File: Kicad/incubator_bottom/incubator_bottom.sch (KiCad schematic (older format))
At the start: 42 parts, among them J1 Conn_01x02, J10 Conn_01x01, J11 Conn_01x01, J12 Conn_01x01, J2 Conn_02x03_Odd_Even, J3 RJ12, J4 Conn_01x01, J5 AudioJack3_SwitchTR, J6 AudioJack3_SwitchTR, J7 Conn_01x01, J8 Conn_01x06, J9 Conn_01x01, Q1 ZXMS6004, Q2 IPB80N03S4L-03, U1 DS18B20Z, U2 DS18B20

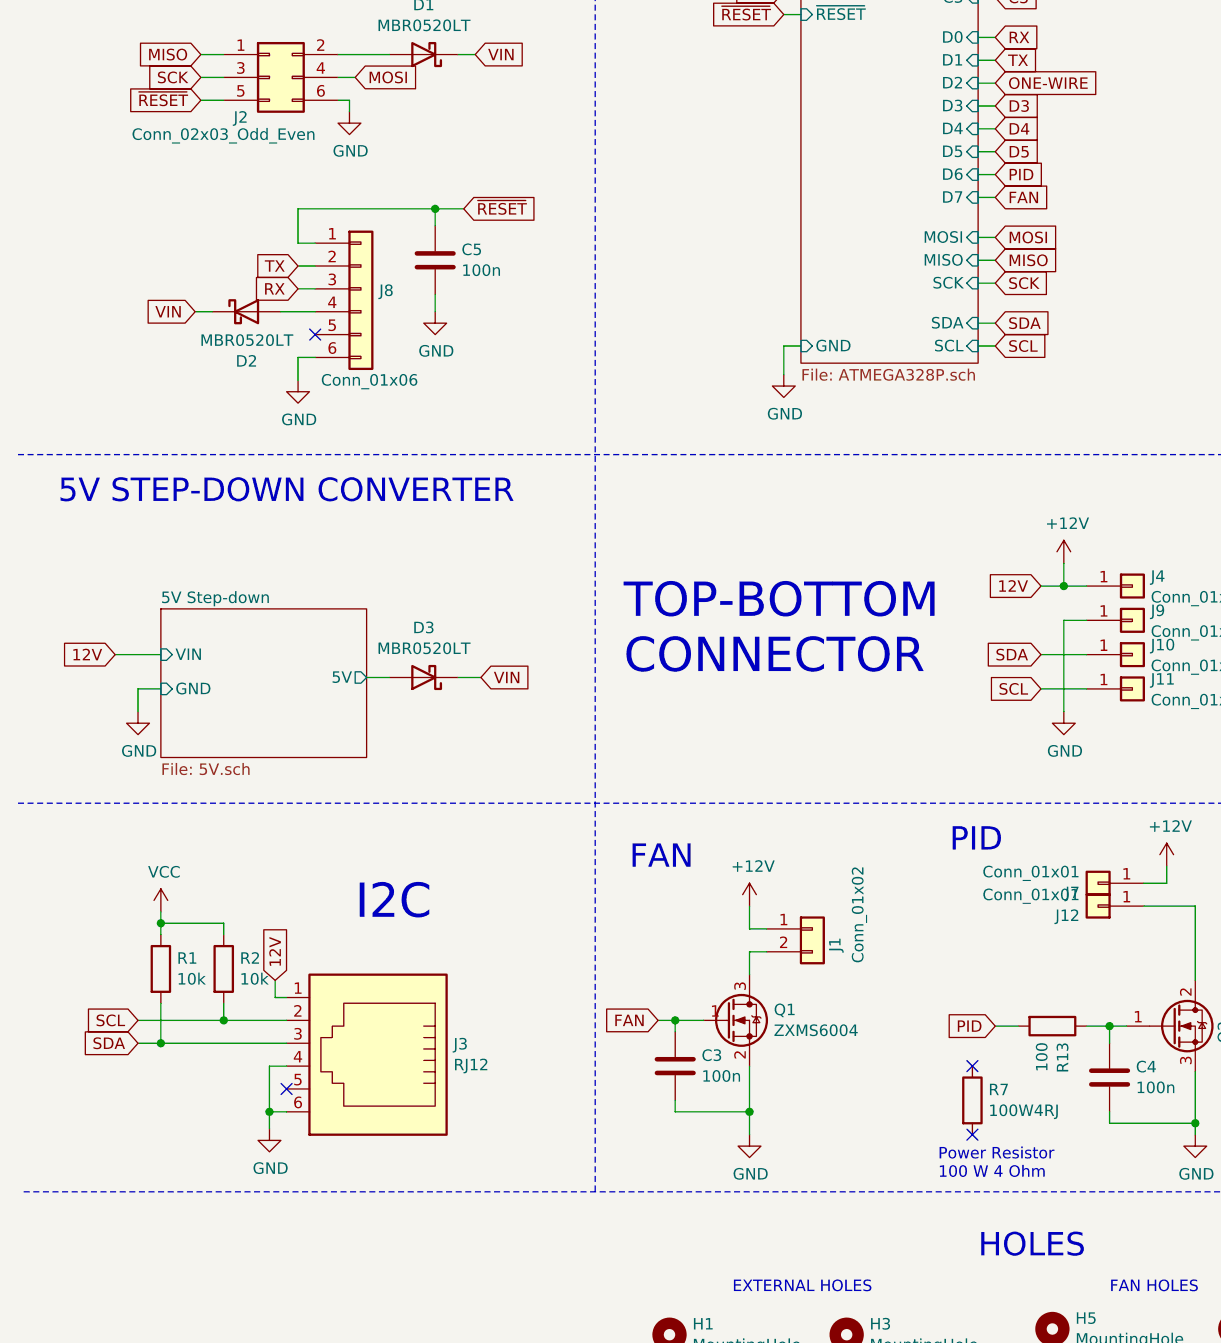
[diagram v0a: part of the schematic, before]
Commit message: refactor: Power supply
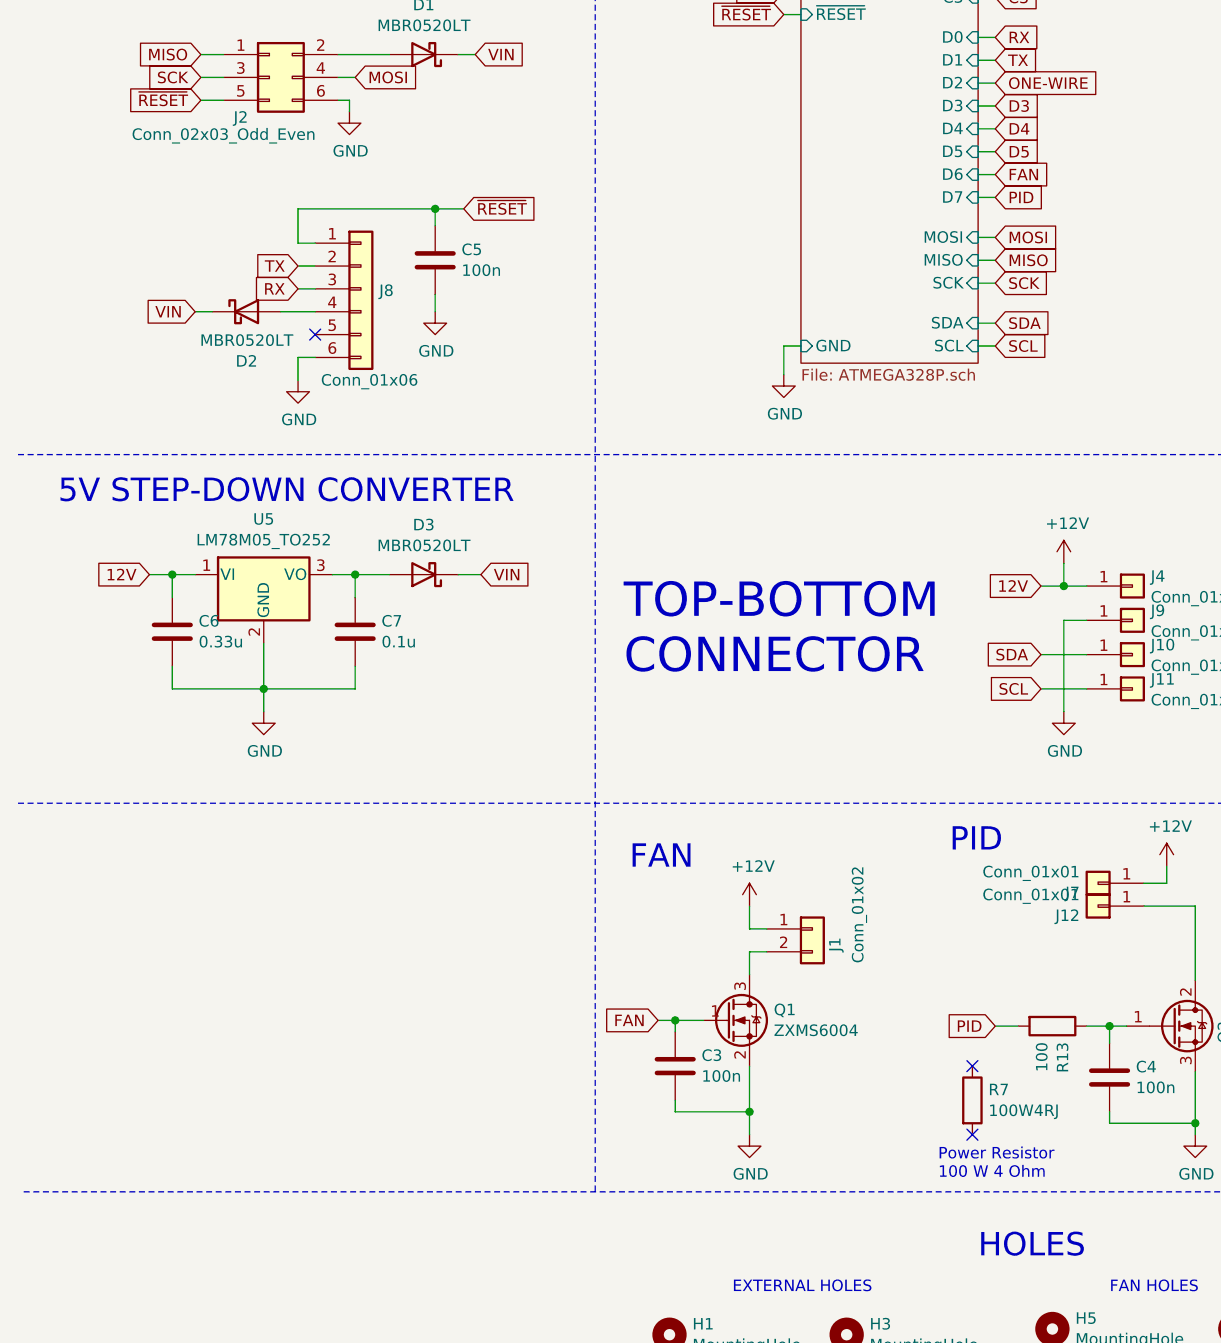
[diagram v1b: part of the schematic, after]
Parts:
- removed J3: RJ12, Incubator:E5566-Q0LK22-L, symbol incubator_bottom-rescue:RJ12-Connector
- removed R1, R2: 10k, Resistor_SMD:R_0805_2012Metric_Pad1.20x1.40mm_HandSolder, symbol incubator_bottom-rescue:R-Device
- added C6: 0.33u, Capacitor_SMD:C_0805_2012Metric_Pad1.18x1.45mm_HandSolder, symbol incubator_bottom-rescue:C-Device
- added C7: 0.1u, Capacitor_SMD:C_0805_2012Metric_Pad1.18x1.45mm_HandSolder, symbol incubator_bottom-rescue:C-Device
- added U5: LM78M05_TO252, Package_TO_SOT_SMD:TO-252-2, symbol Regulator_Linear:LM78M05_TO252
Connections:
- net +12V: now also C6.1, U5.1 (VI)
- net GND: now also C6.2, C7.2, U5.2 (GND)
- net 5V Step-down/5V: no longer names the net of D3.2 (A)
- net 5V Step-down/5V: now also C7.1, U5.3 (VO)
- no-connect marks 8 -> 7
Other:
- note removed: "I2C\n"
- moved on the sheet: D3
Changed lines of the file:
@@
 $Descr A4 11693 8268
 encoding utf-8
-Sheet 1 3
+Sheet 1 2
 Title ""
 Date ""
@@
 C3
 Text GLabel 4750 2200 2    50   Input ~ 0
+PID
+Text GLabel 4750 2100 2    50   Input ~ 0
 FAN
-Text GLabel 4750 2100 2    50   Input ~ 0
-PID
 Text GLabel 4750 2000 2    50   Input ~ 0
 D5
@@
 Text Notes 5250 7000 0    50   ~ 0
 FAN HOLES
-$Sheet
-S 1100 4000 900  650
-U 61425B26
-F0 "5V Step-down" 50
-F1 "5V.sch" 50
-F2 "VIN" I L 1100 4200 50
-F3 "5V" O R 2000 4300 50
-F4 "GND" I L 1100 4350 50
-$EndSheet
-Text GLabel 900  4200 0    50   Input ~ 0
+Text GLabel 1050 3850 0    50   Input ~ 0
 12V
 $Comp
 L incubator_bottom-rescue:GND-power #PWR01
 U 1 1 61433F4F
-P 1000 4450
-F 0 "#PWR01" H 1000 4200 50  0001 C CNN
-F 1 "GND" H 1005 4277 50  0000 C CNN
-F 2 "" H 1000 4450 50  0001 C CNN
-F 3 "" H 1000 4450 50  0001 C CNN
-	1    1000 4450
-	1    0    0    -1
-$EndComp
-Wire Wire Line
-	1000 4450 1000 4350
-Wire Wire Line
-	1000 4350 1100 4350
-Wire Wire Line
-	1100 4200 900  4200
-Text GLabel 2500 4300 2    50   Input ~ 0
+P 1550 4450
+F 0 "#PWR01" H 1550 4200 50  0001 C CNN
+F 1 "GND" H 1555 4277 50  0000 C CNN
+F 2 "" H 1550 4450 50  0001 C CNN
+F 3 "" H 1550 4450 50  0001 C CNN
+	1    1550 4450
+	1    0    0    -1
+$EndComp
+Wire Wire Line
+	1550 4450 1550 4350
+Wire Wire Line
+	1250 3850 1150 3850
+Text GLabel 2500 3850 2    50   Input ~ 0
 VIN
 $Comp
 L incubator_bottom-rescue:MBR0520LT-Diode D3
 U 1 1 61445FAB
-P 2250 4300
-F 0 "D3" H 2250 4083 50  0000 C CNN
-F 1 "MBR0520LT" H 2250 4174 50  0000 C CNN
-F 2 "Diode_SMD:D_SOD-123" H 2250 4125 50  0001 C CNN
-F 3 "http://www.onsemi.com/pub_link/Collateral/MBR0520LT1-D.PDF" H 2250 4300 50  0001 C CNN
-	1    2250 4300
+P 2250 3850
+F 0 "D3" H 2250 3633 50  0000 C CNN
+F 1 "MBR0520LT" H 2250 3724 50  0000 C CNN
+F 2 "Diode_SMD:D_SOD-123" H 2250 3675 50  0001 C CNN
+F 3 "http://www.onsemi.com/pub_link/Collateral/MBR0520LT1-D.PDF" H 2250 3850 50  0001 C CNN
+	1    2250 3850
 	-1   0    0    1
 $EndComp
 Wire Wire Line
-	2500 4300 2400 4300
-Wire Wire Line
-	2100 4300 2000 4300
+	2500 3850 2400 3850
+Wire Wire Line
+	1950 3850 1850 3850
 $Comp
 L Connector_Generic:Conn_01x01 J7
@@
 Text Notes 650  3550 0    102  ~ 0
 5V STEP-DOWN CONVERTER
-Text Notes 1950 5375 0    150  ~ 0
-I2C\n
 Wire Notes Line
 	475  4850 5925 4850
-$Comp
-L incubator_bottom-rescue:RJ12-Connector J3
-U 1 1 610CF354
-P 2050 5900
-F 0 "J3" H 1720 5904 50  0000 R CNN
-F 1 "RJ12" H 1720 5995 50  0000 R CNN
-F 2 "Incubator:E5566-Q0LK22-L" V 2050 5925 50  0001 C CNN
-F 3 "~" V 2050 5925 50  0001 C CNN
-	1    2050 5900
-	-1   0    0    1
-$EndComp
-Text GLabel 1600 5625 1    50   Input ~ 0
-12V
-$Comp
-L incubator_bottom-rescue:R-Device R2
-U 1 1 610DBA03
-P 1375 5575
-F 0 "R2" H 1445 5621 50  0000 L CNN
-F 1 "10k" H 1445 5530 50  0000 L CNN
-F 2 "Resistor_SMD:R_0805_2012Metric_Pad1.20x1.40mm_HandSolder" V 1305 5575 50  0001 C CNN
-F 3 "~" H 1375 5575 50  0001 C CNN
-	1    1375 5575
-	1    0    0    -1
-$EndComp
-$Comp
-L incubator_bottom-rescue:R-Device R1
-U 1 1 610DC2A0
-P 1100 5575
-F 0 "R1" H 1170 5621 50  0000 L CNN
-F 1 "10k" H 1170 5530 50  0000 L CNN
-F 2 "Resistor_SMD:R_0805_2012Metric_Pad1.20x1.40mm_HandSolder" V 1030 5575 50  0001 C CNN
-F 3 "~" H 1100 5575 50  0001 C CNN
-	1    1100 5575
-	1    0    0    -1
-$EndComp
-Wire Wire Line
-	1650 5700 1600 5700
-Wire Wire Line
-	1600 5700 1600 5625
-Text GLabel 1000 5800 0    50   Input ~ 0
-SCL
-Text GLabel 1000 5900 0    50   Input ~ 0
-SDA
-$Comp
-L incubator_bottom-rescue:GND-power #PWR0115
-U 1 1 610DD35E
-P 1575 6275
-F 0 "#PWR0115" H 1575 6025 50  0001 C CNN
-F 1 "GND" H 1580 6102 50  0000 C CNN
-F 2 "" H 1575 6275 50  0001 C CNN
-F 3 "" H 1575 6275 50  0001 C CNN
-	1    1575 6275
-	1    0    0    -1
-$EndComp
-NoConn ~ 1650 6100
-Wire Wire Line
-	1650 6000 1575 6000
-Wire Wire Line
-	1575 6000 1575 6200
-Connection ~ 1575 6200
-Wire Wire Line
-	1650 6200 1575 6200
-Wire Wire Line
-	1575 6200 1575 6275
-Wire Wire Line
-	1650 5900 1100 5900
-Connection ~ 1100 5900
-Wire Wire Line
-	1650 5800 1375 5800
-Connection ~ 1375 5800
-Wire Wire Line
-	1375 5800 1375 5725
-Wire Wire Line
-	1000 5800 1375 5800
-Wire Wire Line
-	1100 5725 1100 5900
-Wire Wire Line
-	1100 5900 1000 5900
-$Comp
-L incubator_bottom-rescue:VCC-power #PWR0114
-U 1 1 610EC2F5
-P 1100 5325
-F 0 "#PWR0114" H 1100 5175 50  0001 C CNN
-F 1 "VCC" H 1115 5498 50  0000 C CNN
-F 2 "" H 1100 5325 50  0001 C CNN
-F 3 "" H 1100 5325 50  0001 C CNN
-	1    1100 5325
-	1    0    0    -1
-$EndComp
-Wire Wire Line
-	1375 5425 1375 5375
-Wire Wire Line
-	1375 5375 1100 5375
-Connection ~ 1100 5375
-Wire Wire Line
-	1100 5375 1100 5325
-Wire Wire Line
-	1100 5425 1100 5375
 Wire Notes Line
 	500  6550 5900 6550
@@
 Text Notes 4500 6500 0    50   ~ 0
 Power Resistor\n100 W 4 Ohm
+$Comp
+L Regulator_Linear:LM78M05_TO252 U5
+U 1 1 6152567E
+P 1550 3850
+F 0 "U5" H 1550 4092 50  0000 C CNN
+F 1 "LM78M05_TO252" H 1550 4001 50  0000 C CNN
+F 2 "Package_TO_SOT_SMD:TO-252-2" H 1550 4075 50  0001 C CIN
+F 3 "https://www.onsemi.com/pub/Collateral/MC78M00-D.PDF" H 1550 3800 50  0001 C CNN
+	1    1550 3850
+	1    0    0    -1
+$EndComp
+$Comp
+L incubator_bottom-rescue:C-Device C6
+U 1 1 61544A4B
+P 1150 4100
+F 0 "C6" H 1265 4146 50  0000 L CNN
+F 1 "0.33u" H 1265 4055 50  0000 L CNN
+F 2 "Capacitor_SMD:C_0805_2012Metric_Pad1.18x1.45mm_HandSolder" H 1188 3950 50  0001 C CNN
+F 3 "~" H 1150 4100 50  0001 C CNN
+	1    1150 4100
+	1    0    0    -1
+$EndComp
+$Comp
+L incubator_bottom-rescue:C-Device C7
+U 1 1 6154606C
+P 1950 4100
+F 0 "C7" H 2065 4146 50  0000 L CNN
+F 1 "0.1u" H 2065 4055 50  0000 L CNN
+F 2 "Capacitor_SMD:C_0805_2012Metric_Pad1.18x1.45mm_HandSolder" H 1988 3950 50  0001 C CNN
+F 3 "~" H 1950 4100 50  0001 C CNN
+	1    1950 4100
+	1    0    0    -1
+$EndComp
+Wire Wire Line
+	1950 3850 1950 3950
+Wire Wire Line
+	2100 3850 1950 3850
+Connection ~ 1950 3850
+Wire Wire Line
+	1150 3950 1150 3850
+Connection ~ 1150 3850
+Wire Wire Line
+	1150 3850 1050 3850
+Wire Wire Line
+	1150 4250 1150 4350
+Wire Wire Line
+	1150 4350 1550 4350
+Connection ~ 1550 4350
+Wire Wire Line
+	1550 4350 1550 4150
+Wire Wire Line
+	1950 4250 1950 4350
+Wire Wire Line
+	1950 4350 1550 4350
 $EndSCHEMATC
